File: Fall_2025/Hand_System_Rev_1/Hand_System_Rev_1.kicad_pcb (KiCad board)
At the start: 2 copper layers, 112.7 x 89.7 mm, 33 parts, among them J1 Barrel_Jack, M1 Motor_Servo, M2 Motor_Servo, M3 Motor_Servo, M4 Motor_Servo, M5 Motor_Servo, M6 Motor_Servo, M7 Stepper_Motor, U1 ESP32-DEVKITC-32UE, U2 LM2596, U3 A4988_Stepper_Motor_Driver, U5 MAX9814ETD_T

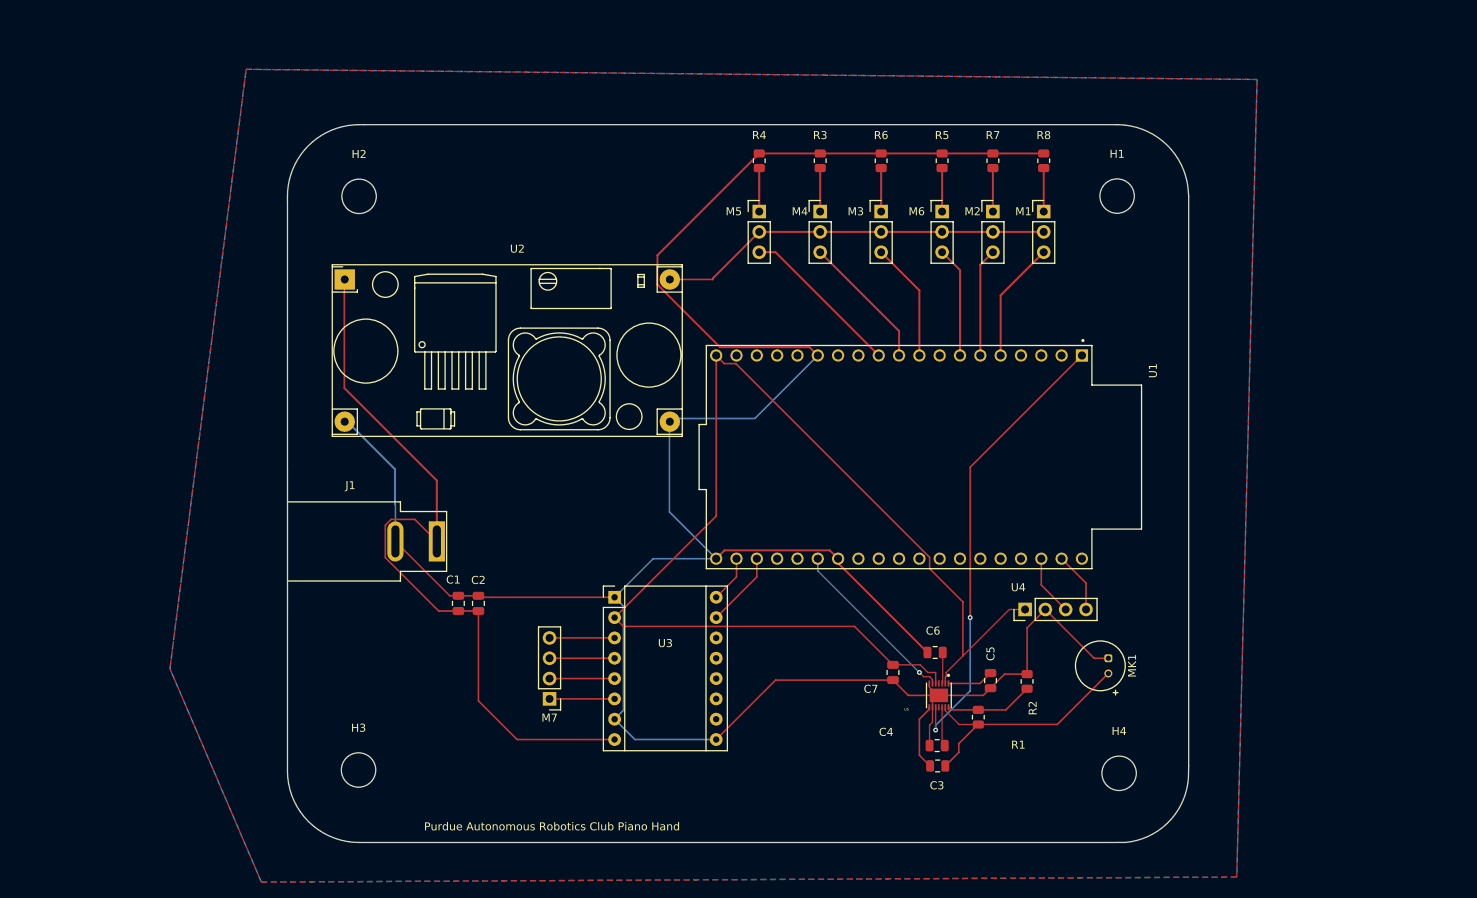
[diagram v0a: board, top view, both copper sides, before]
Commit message: added more stuff
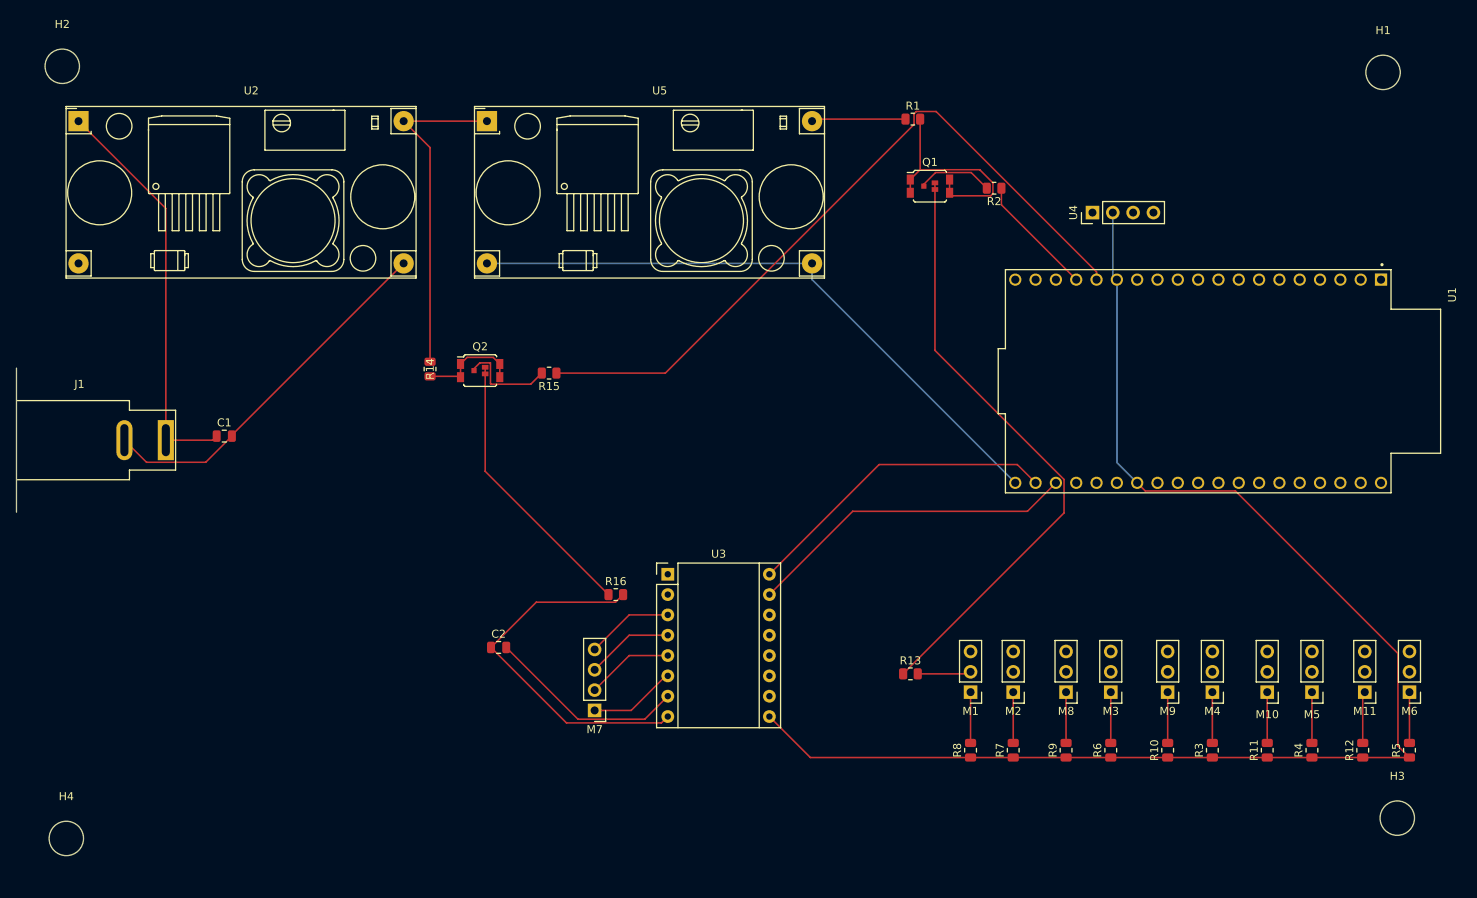
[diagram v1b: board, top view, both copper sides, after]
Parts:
- removed C3: 0.1uF, Capacitor_SMD:C_0805_2012Metric
- removed C4: 0.47uF, Capacitor_SMD:C_0805_2012Metric
- removed C5: 470nF, Capacitor_SMD:C_0805_2012Metric
- removed C6: 2.2uF, Capacitor_SMD:C_0805_2012Metric
- removed C7: 1uF, Capacitor_SMD:C_0805_2012Metric
- removed MK1: Microphone, Sensor_Audio:POM-2244P-C3310-2-R
- added M10: Motor_Servo, Connector_PinHeader_2.54mm:PinHeader_1x03_P2.54mm_Vertical, F.Cu at (215.3, 117.9)
- added M11: Motor_Servo, Connector_PinHeader_2.54mm:PinHeader_1x03_P2.54mm_Vertical, F.Cu at (227.5, 117.9)
- added M8: Motor_Servo, Connector_PinHeader_2.54mm:PinHeader_1x03_P2.54mm_Vertical, F.Cu at (190.1, 117.9)
- added M9: Motor_Servo, Connector_PinHeader_2.54mm:PinHeader_1x03_P2.54mm_Vertical, F.Cu at (202.8, 117.9)
- added Q1: IRF6623, Package_DirectFET:DirectFET_ST, F.Cu at (173.1, 54.6)
- added Q2: IRF6623, Package_DirectFET:DirectFET_ST, F.Cu at (116.9, 77.7)
- added R10: 1K, Resistor_SMD:R_0805_2012Metric, F.Cu at (202.8, 125.1)
- added R11: 1K, Resistor_SMD:R_0805_2012Metric, F.Cu at (215.3, 125.1)
- added R12: 1K, Resistor_SMD:R_0805_2012Metric, F.Cu at (227.2, 125.1)
- added R13: 1k, Resistor_SMD:R_0805_2012Metric, F.Cu at (170.7, 115.6)
- added R14: 10k, Resistor_SMD:R_0805_2012Metric, F.Cu at (110.6, 77.5)
- added R15: 1k, Resistor_SMD:R_0805_2012Metric, F.Cu at (125.5, 78.0)
- added R16: 1k, Resistor_SMD:R_0805_2012Metric, F.Cu at (133.8, 105.7)
- added R9: 1K, Resistor_SMD:R_0805_2012Metric, F.Cu at (190.1, 125.1)
- R1: value 150k -> 10k
- R2: value 100k -> 1k
- U5: value MAX9814ETD_T -> LM2596; footprint MAX9814ETD_T:SON40P300X300X80-15N -> PCB_Components:LM2596
- moved H4 131.9 mm to (65.2, 136.1)
- moved H3 130.0 mm to (231.5, 133.6)
- moved R4 101.0 mm to (220.9, 125.1), turned to 90 degrees
- moved R5 94.0 mm to (233.0, 125.1), turned to 90 degrees
- moved M5 91.6 mm to (220.9, 117.9), turned to 180 degrees
- moved U5 91.3 mm to (117.7, 46.5), turned to 0 degrees
- moved R3 88.5 mm to (208.4, 125.1), turned to 90 degrees
- moved M6 83.8 mm to (233.0, 117.9), turned to 180 degrees
- moved R6 79.1 mm to (195.7, 125.1), turned to 90 degrees
- moved M4 77.5 mm to (208.4, 117.9), turned to 180 degrees
- moved R1 75.2 mm to (171.0, 46.2), turned to 0 degrees
- moved R8 74.2 mm to (178.2, 125.1), turned to 90 degrees
- moved R7 73.7 mm to (183.5, 125.1), turned to 90 degrees
- moved M3 66.6 mm to (195.7, 117.9), turned to 180 degrees
- moved R2 61.8 mm to (181.1, 54.9), turned to 180 degrees
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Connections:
- C1 pad 1: 12V -> 15V
- C2 pad 1: 12V -> STP_P
- J1 pad 1: 12V -> 15V
- M1 pad 2: 7.2V -> MOTOR_P
- M2 pad 2: 7.2V -> MOTOR_P
- M3 pad 2: 7.2V -> MOTOR_P
- M3 pad 3: /INDEX -> /INDEX_2
- M4 pad 2: 7.2V -> MOTOR_P
- M4 pad 3: /MIDDLE -> /MIDDLE_2
- M5 pad 2: 7.2V -> MOTOR_P
- M5 pad 3: /RING -> /RING_2
- M6 pad 2: 7.2V -> MOTOR_P
- M6 pad 3: /PINKIE -> /PINKIE_2
- R1 pad 1: Net-(MK1-+) -> 7.2V
- R1 pad 2: Net-(U5-TH) -> Net-(Q1-D)
- R2 pad 1: Net-(U5-TH) -> /SERVO_VG
- R2 pad 2: GND -> Net-(Q1-G)
- U1 pad 10: /MIDDLE -> unconnected-(U1-26-Pad10)
- U1 pad 11: /RING -> unconnected-(U1-27-Pad11)
- U1 pad 12: unconnected-(U1-14-Pad12) -> /DT
- U1 pad 13: unconnected-(U1-12-Pad13) -> /CW
- U1 pad 15: unconnected-(U1-13-Pad15) -> /STP_VG
- U1 pad 16: unconnected-(U1-D2-Pad16) -> /SERVO_VG
- U1 pad 23: unconnected-(U1-TX-Pad23) -> /THUMB_1
- U1 pad 24: unconnected-(U1-RX-Pad24) -> /THUMB_2
- U1 pad 25: /MP_OUT -> /INDEX_1
- U1 pad 27: unconnected-(U1-19-Pad27) -> /INDEX_2
- U1 pad 28: unconnected-(U1-18-Pad28) -> /MIDDLE_1
- U1 pad 29: unconnected-(U1-5-Pad29) -> /MIDDLE_2
- U1 pad 30: unconnected-(U1-17-Pad30) -> /RING_1
- U1 pad 31: unconnected-(U1-16-Pad31) -> /RING_2
- U1 pad 32: unconnected-(U1-4-Pad32) -> /PINKIE_1
- U1 pad 33: unconnected-(U1-0-Pad33) -> /PINKIE_2
- U1 pad 36: /CW -> unconnected-(U1-D1-Pad36)
- U1 pad 37: /DT -> unconnected-(U1-D0-Pad37)
- U1 pad 5: /THUMB_1 -> unconnected-(U1-34-Pad5)
- U1 pad 6: /THUMB_2 -> unconnected-(U1-35-Pad6)
- U1 pad 7: /PINKIE -> unconnected-(U1-32-Pad7)
- U1 pad 9: /INDEX -> unconnected-(U1-25-Pad9)
- U2 pad 1: 12V -> 15V
- U2 pad 4: 7.2V -> 12V
- U3 pad 8: 12V -> STP_P
- U5 pad 1: Net-(U5-CT) -> 12V
- U5 pad 2: 5V -> GND
- U5 pad 3: Net-(U5-CG) -> GND
- U5 pad 4: (no net) -> 7.2V
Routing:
- net /STP_VG: track 0.00 -> 91.1 mm
- net Net-(Q1-S): track 0.00 -> 76.4 mm
- net GND: track 320.7 -> 386.5 mm
- net 5V: track 148.1 -> 86.0 mm
- net MOTOR_P: track 0.00 -> 61.6 mm
- net 3.3V: track 57.3 -> 0.00 mm, vias 2 -> 0
- net 12V: track 94.5 -> 41.9 mm
- net 15V: track 0.00 -> 51.0 mm
- net STP_P: track 0.00 -> 45.6 mm
- net 7.2V: track 49.3 -> 11.8 mm
- net Net-(Q2-S): track 0.00 -> 34.8 mm
- net /DIR_PIN: track 5.88 -> 39.9 mm
- net /STEP_PIN: track 9.47 -> 41.6 mm
- net Net-(MK1-+): track 31.1 -> 0.00 mm
- net Net-(Q1-D): track 0.00 -> 28.2 mm
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- removed copper zone on B.Cu, net GND
- removed copper zone on F.Cu, net GND
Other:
- board outline removed
- copper layers 2 -> 4
- board text removed: "Purdue Autonomous Robotics Club Piano Hand"

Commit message: more stuff for organizing into spring 2026
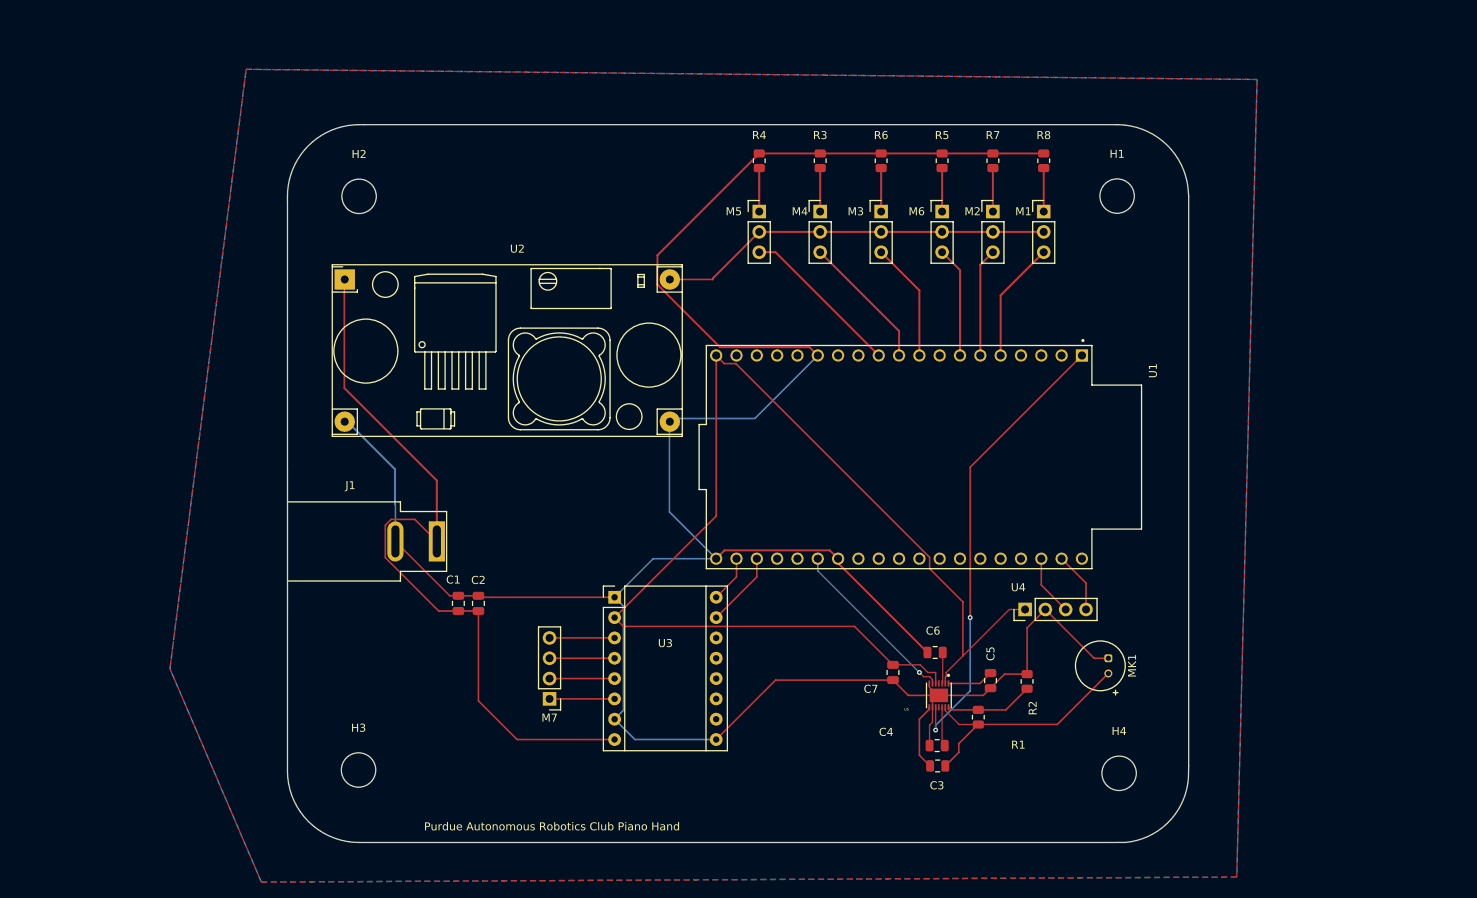
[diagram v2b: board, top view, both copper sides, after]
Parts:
- removed M10, M11, M8, M9: Motor_Servo, Connector_PinHeader_2.54mm:PinHeader_1x03_P2.54mm_Vertical
- removed Q1, Q2: IRF6623, Package_DirectFET:DirectFET_ST
- removed R10, R11, R12, R9: 1K, Resistor_SMD:R_0805_2012Metric
- removed R13, R15, R16: 1k, Resistor_SMD:R_0805_2012Metric
- removed R14: 10k, Resistor_SMD:R_0805_2012Metric
- added C3: 0.1uF, Capacitor_SMD:C_0805_2012Metric, F.Cu at (174.1, 127.1)
- added C4: 0.47uF, Capacitor_SMD:C_0805_2012Metric, F.Cu at (174.0, 124.5)
- added C5: 470nF, Capacitor_SMD:C_0805_2012Metric, F.Cu at (180.7, 116.4)
- added C6: 2.2uF, Capacitor_SMD:C_0805_2012Metric, F.Cu at (173.8, 112.9)
- added C7: 1uF, Capacitor_SMD:C_0805_2012Metric, F.Cu at (168.5, 115.4)
- added MK1: Microphone, Sensor_Audio:POM-2244P-C3310-2-R, F.Cu at (195.4, 113.6)
- R1: value 10k -> 150k
- R2: value 1k -> 100k
- U5: value LM2596 -> MAX9814ETD_T; footprint PCB_Components:LM2596 -> MAX9814ETD_T:SON40P300X300X80-15N
- moved H4 131.9 mm to (196.8, 128.0)
- moved H3 130.0 mm to (101.7, 127.6)
- moved R4 101.0 mm to (151.8, 51.4), turned to -90 degrees
- moved R5 94.0 mm to (174.6, 51.4), turned to -90 degrees
- moved M5 91.6 mm to (151.8, 57.8), turned to 0 degrees
- moved U5 91.3 mm to (174.2, 118.3), turned to -90 degrees
- moved R3 88.5 mm to (159.4, 51.4), turned to -90 degrees
- moved M6 83.8 mm to (174.6, 57.8), turned to 0 degrees
- moved R6 79.1 mm to (167.0, 51.4), turned to -90 degrees
- moved M4 77.5 mm to (159.4, 57.8), turned to 0 degrees
- moved R1 75.2 mm to (179.2, 121.0), turned to 90 degrees
- moved R8 74.2 mm to (187.3, 51.4), turned to -90 degrees
- moved R7 73.7 mm to (181.0, 51.4), turned to -90 degrees
- moved M3 66.6 mm to (167.0, 57.8), turned to 0 degrees
- moved R2 61.8 mm to (185.2, 116.5), turned to 90 degrees
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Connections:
- C1 pad 1: 15V -> 12V
- C2 pad 1: STP_P -> 12V
- J1 pad 1: 15V -> 12V
- M1 pad 2: MOTOR_P -> 7.2V
- M2 pad 2: MOTOR_P -> 7.2V
- M3 pad 2: MOTOR_P -> 7.2V
- M3 pad 3: /INDEX_2 -> /INDEX
- M4 pad 2: MOTOR_P -> 7.2V
- M4 pad 3: /MIDDLE_2 -> /MIDDLE
- M5 pad 2: MOTOR_P -> 7.2V
- M5 pad 3: /RING_2 -> /RING
- M6 pad 2: MOTOR_P -> 7.2V
- M6 pad 3: /PINKIE_2 -> /PINKIE
- R1 pad 1: 7.2V -> Net-(MK1-+)
- R1 pad 2: Net-(Q1-D) -> Net-(U5-TH)
- R2 pad 1: /SERVO_VG -> Net-(U5-TH)
- R2 pad 2: Net-(Q1-G) -> GND
- U1 pad 10: unconnected-(U1-26-Pad10) -> /MIDDLE
- U1 pad 11: unconnected-(U1-27-Pad11) -> /RING
- U1 pad 12: /DT -> unconnected-(U1-14-Pad12)
- U1 pad 13: /CW -> unconnected-(U1-12-Pad13)
- U1 pad 15: /STP_VG -> unconnected-(U1-13-Pad15)
- U1 pad 16: /SERVO_VG -> unconnected-(U1-D2-Pad16)
- U1 pad 23: /THUMB_1 -> unconnected-(U1-TX-Pad23)
- U1 pad 24: /THUMB_2 -> unconnected-(U1-RX-Pad24)
- U1 pad 25: /INDEX_1 -> /MP_OUT
- U1 pad 27: /INDEX_2 -> unconnected-(U1-19-Pad27)
- U1 pad 28: /MIDDLE_1 -> unconnected-(U1-18-Pad28)
- U1 pad 29: /MIDDLE_2 -> unconnected-(U1-5-Pad29)
- U1 pad 30: /RING_1 -> unconnected-(U1-17-Pad30)
- U1 pad 31: /RING_2 -> unconnected-(U1-16-Pad31)
- U1 pad 32: /PINKIE_1 -> unconnected-(U1-4-Pad32)
- U1 pad 33: /PINKIE_2 -> unconnected-(U1-0-Pad33)
- U1 pad 36: unconnected-(U1-D1-Pad36) -> /CW
- U1 pad 37: unconnected-(U1-D0-Pad37) -> /DT
- U1 pad 5: unconnected-(U1-34-Pad5) -> /THUMB_1
- U1 pad 6: unconnected-(U1-35-Pad6) -> /THUMB_2
- U1 pad 7: unconnected-(U1-32-Pad7) -> /PINKIE
- U1 pad 9: unconnected-(U1-25-Pad9) -> /INDEX
- U2 pad 1: 15V -> 12V
- U2 pad 4: 12V -> 7.2V
- U3 pad 8: STP_P -> 12V
- U5 pad 1: 12V -> Net-(U5-CT)
- U5 pad 2: GND -> 5V
- U5 pad 3: GND -> Net-(U5-CG)
- U5 pad 4: 7.2V -> (no net)
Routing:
- net /STP_VG: track 91.1 -> 0.00 mm
- net Net-(Q1-S): track 76.4 -> 0.00 mm
- net GND: track 386.5 -> 320.7 mm
- net 5V: track 86.0 -> 148.1 mm
- net MOTOR_P: track 61.6 -> 0.00 mm
- net 3.3V: track 0.00 -> 57.3 mm, vias 0 -> 2
- net 12V: track 41.9 -> 94.5 mm
- net 15V: track 51.0 -> 0.00 mm
- net STP_P: track 45.6 -> 0.00 mm
- net 7.2V: track 11.8 -> 49.3 mm
- net Net-(Q2-S): track 34.8 -> 0.00 mm
- net /DIR_PIN: track 39.9 -> 5.88 mm
- net /STEP_PIN: track 41.6 -> 9.47 mm
- net Net-(MK1-+): track 0.00 -> 31.1 mm
- net Net-(Q1-D): track 28.2 -> 0.00 mm
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- added copper zone on B.Cu, net GND
- added copper zone on F.Cu, net GND
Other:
- board outline added: 112.7 x 89.7 mm
- copper layers 4 -> 2
- board text added: "Purdue Autonomous Robotics Club Piano Hand"
